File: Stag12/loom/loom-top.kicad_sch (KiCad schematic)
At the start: 3 parts

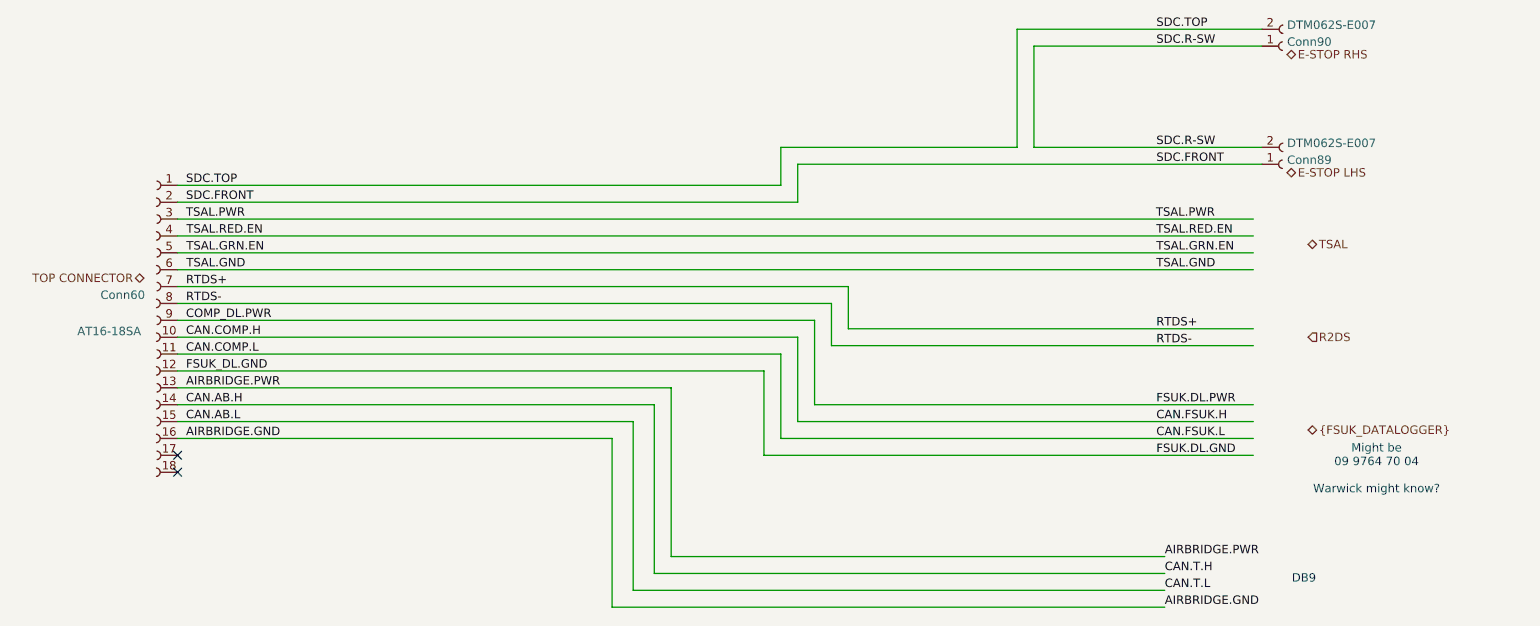
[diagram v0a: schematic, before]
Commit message: TSAL pinout
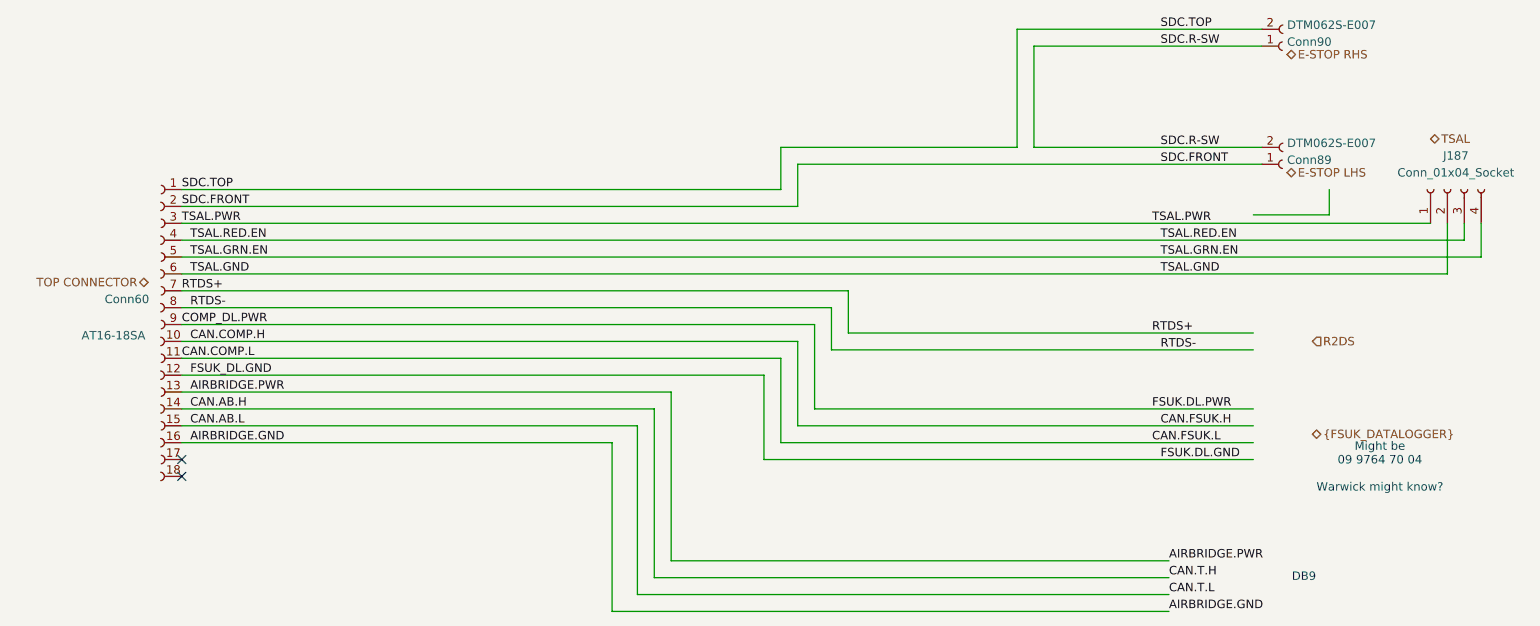
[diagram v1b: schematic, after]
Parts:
- added J187: Conn_01x04_Socket, symbol Connector:Conn_01x04_Socket
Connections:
- net TSAL.GND: now also J187.2 (Pin_2)
- net TSAL.GRN.EN: now also J187.4 (Pin_4)
- net TSAL.PWR: now also J187.1 (Pin_1)
- net TSAL.RED.EN: now also J187.3 (Pin_3)
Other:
- moved on the sheet: Conn60
